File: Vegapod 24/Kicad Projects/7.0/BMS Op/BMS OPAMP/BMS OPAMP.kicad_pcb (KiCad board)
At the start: 2 copper layers, 85.1 x 85.1 mm, 142 parts, among them J1 CHG/DSCHG CTRL, J2 CHG/DSCHG CTRL CMP (SHORT DAT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, J3 Data IN/OUT, J4 Data IN/OUT, J5 Port Selector, J6 Port Selector, J7 NTC1, J8 NTC2, J9 Balance Connector, Q1 MMBT3906, Q2 MMBT3904, Q3 MMBT3904, Q4 MMBT3904, Q5 MMBT3904, Q6 MMBT3904, Q7 MMBT3904, U1 TLP185, U10 LM324, U11 LM324, U2 TLP185, U3 TLP185, U4 TLP185, U5 TLP185, U6 6N137, U7 6N137, U8 LM78M05_TO252, U9 LM324

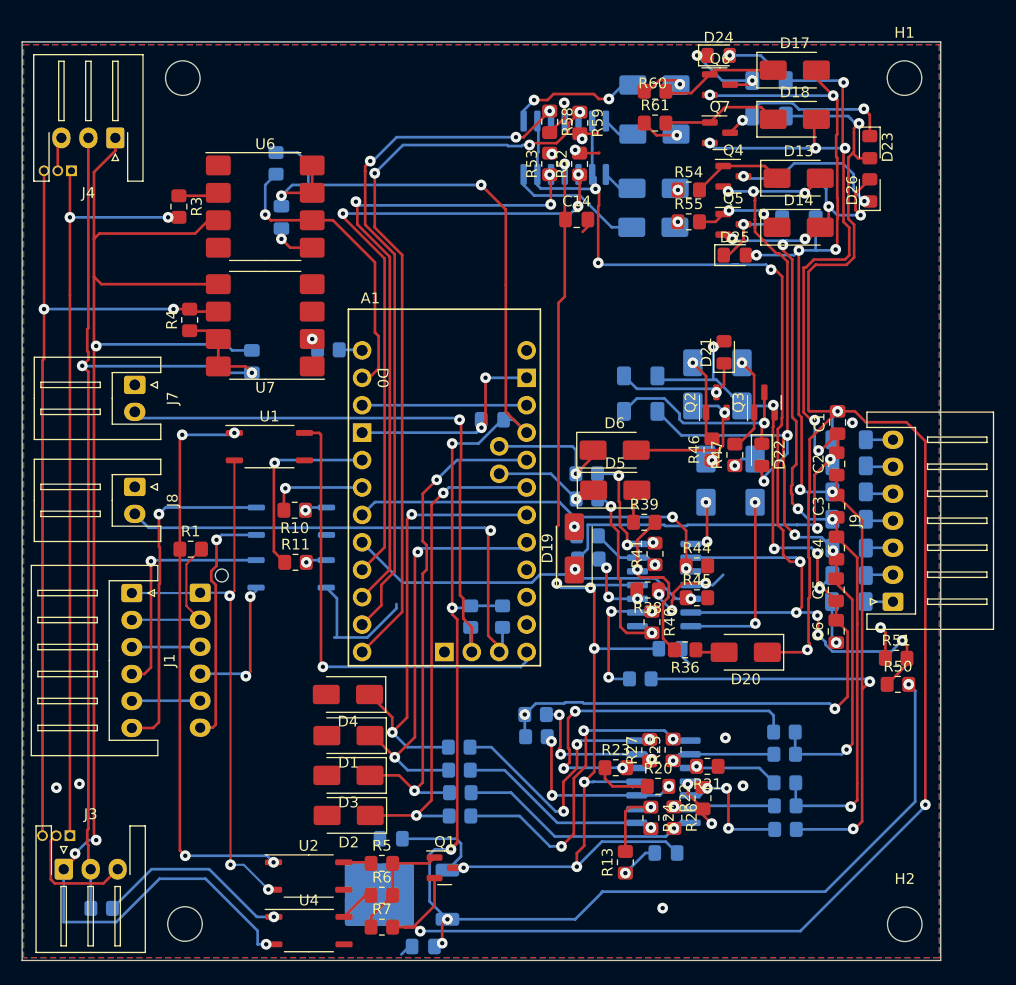
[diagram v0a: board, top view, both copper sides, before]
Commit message: Almost complete bms slave
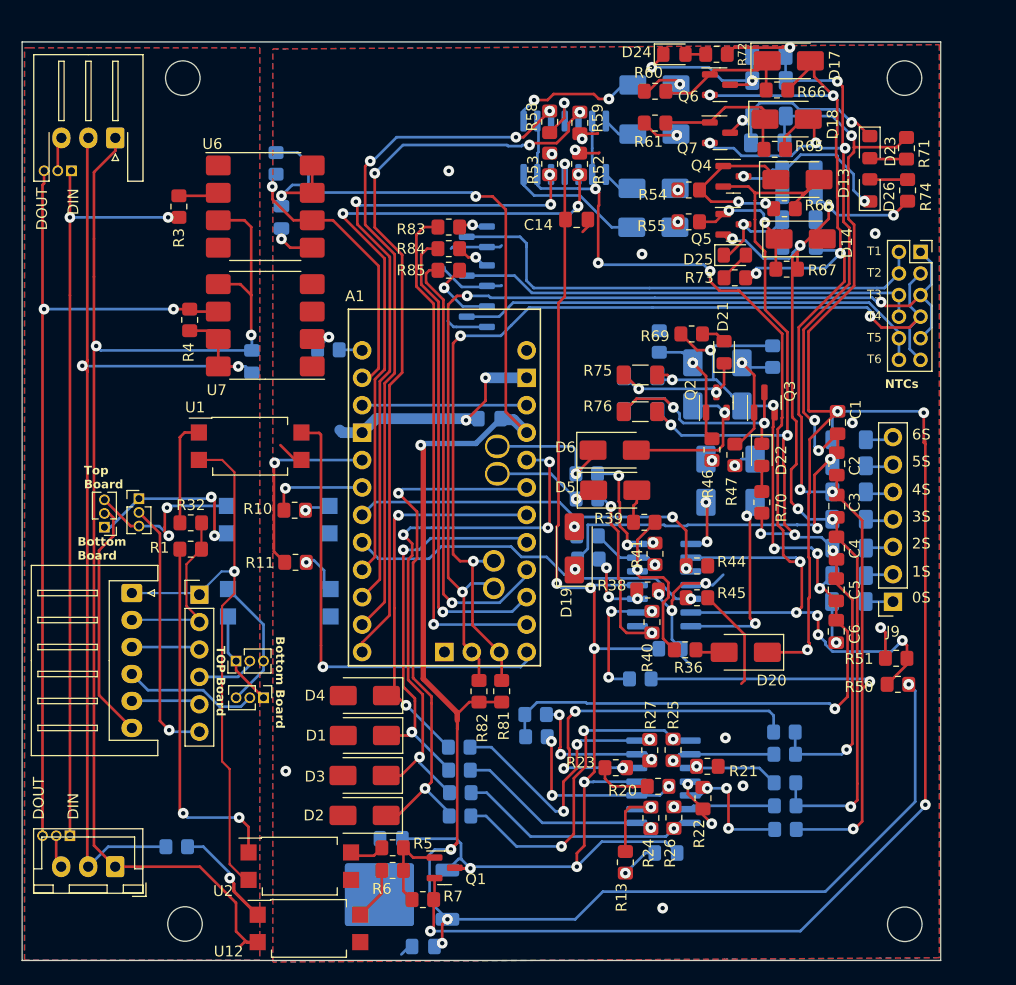
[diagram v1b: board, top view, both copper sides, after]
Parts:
- removed U5: TLP185, Package_SO:SOIC-4_4.55x3.7mm_P2.54mm
- added J10: Port Selector, Connector_PinHeader_1.27mm:PinHeader_1x03_P1.27mm_Vertical, F.Cu at (44.8, 76.5)
- added J11: Port Selector, Connector_PinHeader_1.27mm:PinHeader_1x03_P1.27mm_Vertical, F.Cu at (42.3, 73.1)
- added J18: Conn_02x06_Odd_Even, Connector_PinSocket_2.00mm:PinSocket_2x06_P2.00mm_Vertical, F.Cu at (105.7, 35.2)
- added Q10: MMBT3904/AM2304/AO3400, Package_TO_SOT_SMD:SOT-23, B.Cu at (64.6, 41.2)
- added Q8: MMBT3904/AM2304/AO3400, Package_TO_SOT_SMD:SOT-23, B.Cu at (64.6, 33.8)
- added Q9: MMBT3904/AM2304/AO3400, Package_TO_SOT_SMD:SOT-23, B.Cu at (64.6, 37.4)
- added R64: 47K, Resistor_SMD:R_0805_2012Metric_Pad1.20x1.40mm_HandSolder, B.Cu at (92.0, 44.9)
- added R65: 47K, Resistor_SMD:R_0805_2012Metric_Pad1.20x1.40mm_HandSolder, F.Cu at (92.2, 25.7)
- added R66: 47K, Resistor_SMD:R_0805_2012Metric_Pad1.20x1.40mm_HandSolder, F.Cu at (92.4, 20.2)
- added R67: 47K, Resistor_SMD:R_0805_2012Metric_Pad1.20x1.40mm_HandSolder, F.Cu at (93.3, 36.8)
- added R68: 47K, Resistor_SMD:R_0805_2012Metric_Pad1.20x1.40mm_HandSolder, F.Cu at (93.1, 31.2)
- added R69: 470, Resistor_SMD:R_0805_2012Metric_Pad1.20x1.40mm_HandSolder, F.Cu at (84.5, 42.8)
- added R70: 470, Resistor_SMD:R_0805_2012Metric_Pad1.20x1.40mm_HandSolder, F.Cu at (91.0, 58.4)
- added R71: 470, Resistor_SMD:R_0805_2012Metric_Pad1.20x1.40mm_HandSolder, F.Cu at (104.4, 25.6)
- added R72: 470, Resistor_SMD:R_0805_2012Metric_Pad1.20x1.40mm_HandSolder, F.Cu at (86.8, 16.9)
- added R73: 470, Resistor_SMD:R_0805_2012Metric_Pad1.20x1.40mm_HandSolder, F.Cu at (88.5, 37.6)
- added R74: 470, Resistor_SMD:R_0805_2012Metric_Pad1.20x1.40mm_HandSolder, F.Cu at (104.5, 29.5)
- added R75: 33, Resistor_SMD:R_1206_3216Metric_Pad1.30x1.75mm_HandSolder, F.Cu at (79.8, 46.6)
- added R76: 33, Resistor_SMD:R_1206_3216Metric_Pad1.30x1.75mm_HandSolder, F.Cu at (79.8, 50.0)
- added R77: 33, Resistor_SMD:R_1206_3216Metric_Pad1.30x1.75mm_HandSolder, B.Cu at (91.5, 25.1)
- added R78: 33, Resistor_SMD:R_1206_3216Metric_Pad1.30x1.75mm_HandSolder, B.Cu at (91.7, 17.0)
- added R79: 33, Resistor_SMD:R_1206_3216Metric_Pad1.30x1.75mm_HandSolder, B.Cu at (94.5, 34.6)
- added R80: 33, Resistor_SMD:R_1206_3216Metric_Pad1.30x1.75mm_HandSolder, B.Cu at (94.5, 29.9)
- added R81: 4.7k, Resistor_SMD:R_0805_2012Metric_Pad1.20x1.40mm_HandSolder, F.Cu at (66.9, 75.9)
- added R82: 4.7k, Resistor_SMD:R_0805_2012Metric_Pad1.20x1.40mm_HandSolder, F.Cu at (64.8, 75.9)
- added R83: 470, Resistor_SMD:R_0805_2012Metric_Pad1.20x1.40mm_HandSolder, F.Cu at (62.0, 32.9)
- added R84: 470, Resistor_SMD:R_0805_2012Metric_Pad1.20x1.40mm_HandSolder, F.Cu at (62.0, 34.9)
- added R85: 470, Resistor_SMD:R_0805_2012Metric_Pad1.20x1.40mm_HandSolder, F.Cu at (62.0, 36.9)
- added U12: PC817, Package_SO:SSO-4_6.7x5.1mm_P2.54mm_Clearance8mm, F.Cu at (49.0, 97.9)
- D10, D13, D14, D17, D18, D9: value 1n4007 -> 12V Z
- D11, D12, D15, D16, D7, D8: value 1n4007 -> M7
- D19, D20: value 5.1V Z -> Short It Out
- J2: footprint Connector_JST:JST_XH_B6B-XH-AM_1x06_P2.50mm_Vertical -> Connector_PinHeader_2.54mm:PinHeader_1x06_P2.54mm_Vertical; moved to F.Cu
- J3: footprint Connector_JST:JST_XH_S3B-XH-A-1_1x03_P2.50mm_Horizontal -> Connector_JST:JST_XH_B3B-XH-A_1x03_P2.50mm_Vertical
- J7: value NTC1 -> Port Selector; footprint Connector_JST:JST_XH_S2B-XH-A_1x02_P2.50mm_Horizontal -> Connector_PinHeader_1.27mm:PinHeader_1x03_P1.27mm_Vertical
- J8: value NTC2 -> Port Selector; footprint Connector_JST:JST_XH_S2B-XH-A_1x02_P2.50mm_Horizontal -> Connector_PinHeader_1.27mm:PinHeader_1x03_P1.27mm_Vertical
- J9: footprint Connector_JST:JST_XH_S7B-XH-A_1x07_P2.50mm_Horizontal -> Connector_PinSocket_2.54mm:PinSocket_1x07_P2.54mm_Vertical
- Q1: value MMBT3906 -> MMBT3906/FDN358P
- Q2, Q3, Q4, Q5, Q6, Q7: value MMBT3904 -> MMBT3904/AM2304/AO3400
- R1: value 330 -> 470
- R12, R14, R15, R16, R17, R18, R19, R21, R22, R23, R25, R26, R27, R34, R35, R36, R37, R38, R39, R40, R41, R44, R45, R52, R53, R58, R59: value 10k -> 47K
- R13, R20, R24: value 10k -> 47k
- R28, R29, R30, R31, R42, R43: value 10k -> 470
- R32: value 1k -> 470; moved to F.Cu
- R33: value 1k -> 47K
- R46, R47, R50, R51, R54, R55, R60: value 1k -> 470
- R61: value 1k -> SHORT OUT
- U1, U2, U3: value TLP185 -> PC817; footprint Package_SO:SOIC-4_4.55x3.7mm_P2.54mm -> Package_SO:SSO-4_6.7x5.1mm_P2.54mm_Clearance8mm
- U4: value TLP185 -> PC817; footprint Package_SO:SOIC-4_4.55x3.7mm_P2.54mm -> Package_SO:SSO-4_6.7x5.1mm_P2.54mm_Clearance8mm; moved to B.Cu
- moved U4 30.5 mm to (46.3, 67.7), turned to 180 degrees
- moved R33 29.3 mm to (81.5, 43.5)
- moved R32 27.3 mm to (38.1, 60.3), turned to 0 degrees
- moved J7 13.5 mm to (30.1, 60.7), turned to 180 degrees
- moved R2 9.00 mm to (36.8, 90.3)
- moved J3 4.78 mm to (31.1, 92.2), turned to 180 degrees
- moved R7 4.57 mm to (59.6, 95.2)
- moved D24 4.10 mm to (82.9, 16.9)
- moved R6 2.50 mm to (56.8, 92.5)
- moved U1 1.79 mm to (43.6, 53.2)
- moved R5 1.76 mm to (56.8, 90.4)
- moved D4 1.57 mm to (54.2, 76.3)
- moved D1 1.52 mm to (54.2, 80.0)
- moved D3 1.50 mm to (54.2, 83.7)
- moved D2 1.47 mm to (54.2, 87.4)
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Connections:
- A1 pad D11: unconnected-(A1-D11_MOSI-PadD11) -> DTEMP1
- A1 pad D12: unconnected-(A1-D12_MISO-PadD12) -> DTEMP2
- A1 pad D13: unconnected-(A1-D13_SCK-PadD13) -> DTEMP3
- D21 pad 2: B1 -> Net-(D21-A)
- D22 pad 2: B2 -> Net-(D22-A)
- D23 pad 2: B6 -> Net-(D23-A)
- D24 pad 2: B5 -> Net-(D24-A)
- D25 pad 2: B4 -> Net-(D25-A)
- D26 pad 2: B3 -> Net-(D26-A)
- J7 pad 1: B0 -> Net-(J7-Pin_1)
- J7 pad 2: A6 -> Net-(J1-Pin_6)
- J8 pad 1: B0 -> Net-(J7-Pin_1)
- J8 pad 2: A7 -> Net-(J2-Pin_6)
- R32 pad 1: 5V -> Net-(R32-Pad1)
- R32 pad 2: A6 -> CHGDT+
- R33 pad 1: 5V -> B0
- R33 pad 2: A7 -> Net-(D9-K)
- U1 pad 1: Net-(R1-Pad1) -> Net-(R32-Pad1)
- U1 pad 3: CHGDT- -> B0
- U1 pad 4: B0 -> DCHG
- U2 pad 3: CHGDT- -> B0
- U2 pad 4: B0 -> Net-(R5-Pad1)
- U3 pad 3: B0 -> Net-(J7-Pin_1)
- U3 pad 4: Net-(J2-Pin_6) -> Net-(J7-Pin_3)
- U4 pad 1: Net-(R2-Pad1) -> Net-(R11-Pad2)
- U4 pad 3: DIN_GND -> Net-(J10-Pin_1)
- U4 pad 4: B0 -> Net-(J10-Pin_3)
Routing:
- net DTEMP1: track 0.00 -> 47.9 mm, vias 0 -> 1
- net NTC_GND1: track 0.00 -> 46.6 mm
- net A7: track 47.8 -> 92.8 mm, vias 1 -> 3
- net NTC_GND3: track 0.00 -> 44.3 mm
- net DTEMP2: track 0.00 -> 44.0 mm, vias 0 -> 1
- net NTC_GND2: track 0.00 -> 42.8 mm
- net DTEMP3: track 0.00 -> 41.2 mm, vias 0 -> 1
- net A6: track 54.8 -> 93.9 mm, vias 1 -> 3
- net B0: track 100.5 -> 122.3 mm, vias 22 -> 24
- net Net-(R1-Pad1): track 52.6 -> 34.2 mm, vias 4 -> 2
- net DIN_GND: track 138.3 -> 122.2 mm, vias 4 -> 2
- net Net-(J7-Pin_1): track 0.00 -> 16.0 mm, vias 0 -> 2
- net Net-(J7-Pin_3): track 0.00 -> 15.9 mm, vias 0 -> 2
- net Net-(J10-Pin_3): track 0.00 -> 12.9 mm
- net B4: track 128.0 -> 138.0 mm, vias 9 -> 8
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- added copper zone on B.Cu, net DIN_GND
- added copper zone on F.Cu, net DIN_GND
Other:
- board text added: "."
- board text added: "0S"
- board text added: "1S"
- board text added: "2S"
- board text added: "3S"
- board text added: "4S"
- board text added: "5S"
- board text added: "6S"
- board text added: "Bottom Board"
- board text added: "DIN"
- board text added: "DOUT"
- board text added: "NTCs"
- board text added: "T1"
- board text added: "T2"
- board text added: "T3"
- board text added: "T4"
- board text added: "T5"
- board text added: "T6"
- board text added: "TOP Board"
- board text added: "Top Board"
